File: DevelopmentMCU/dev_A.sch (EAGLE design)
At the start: 9 parts, among them U1 TM4C123_DEVICE

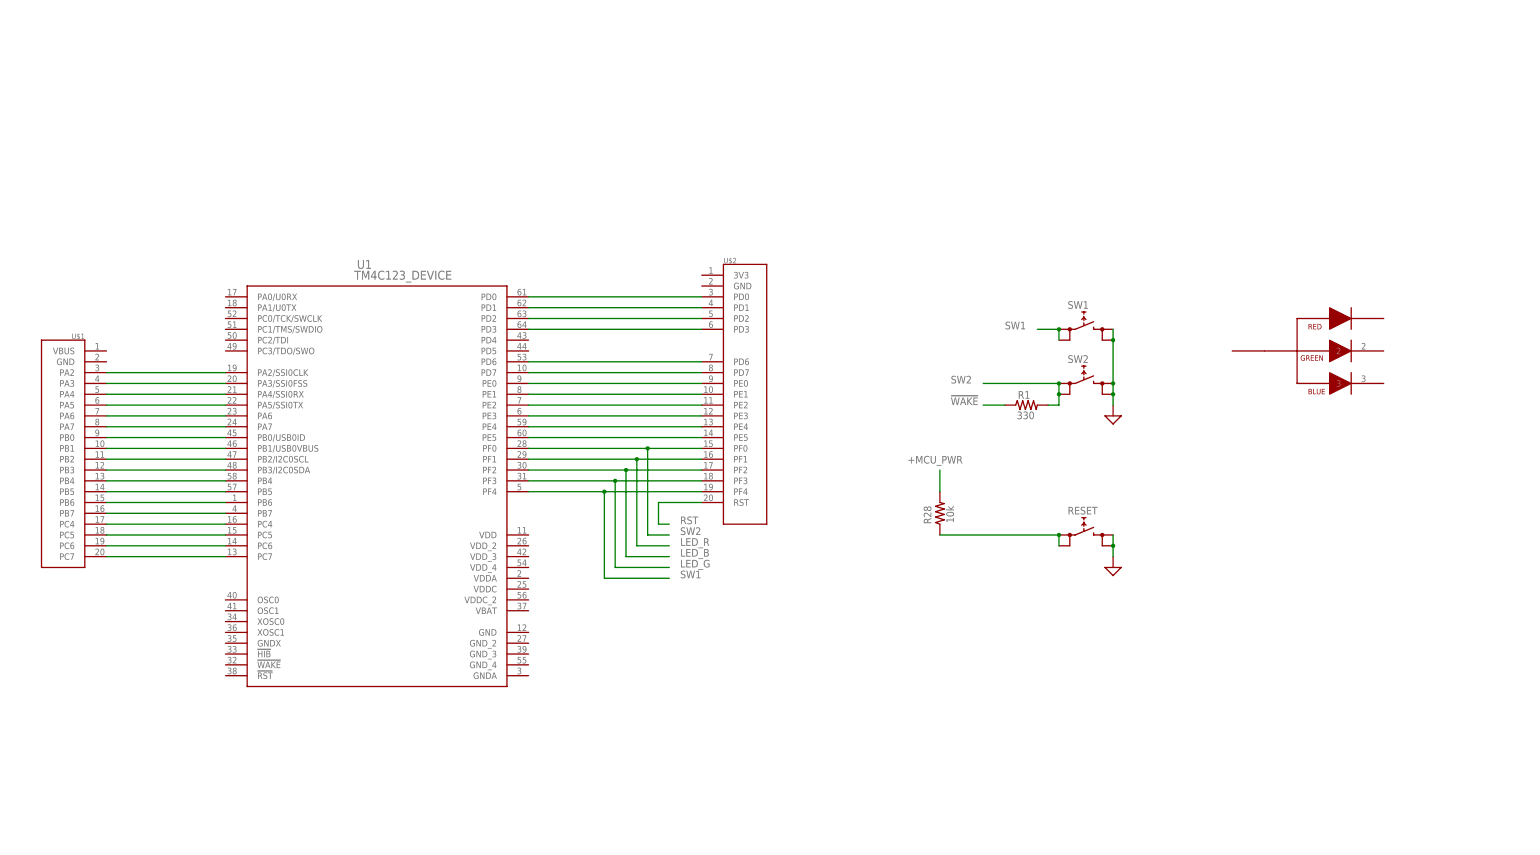
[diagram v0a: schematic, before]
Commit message: Staging
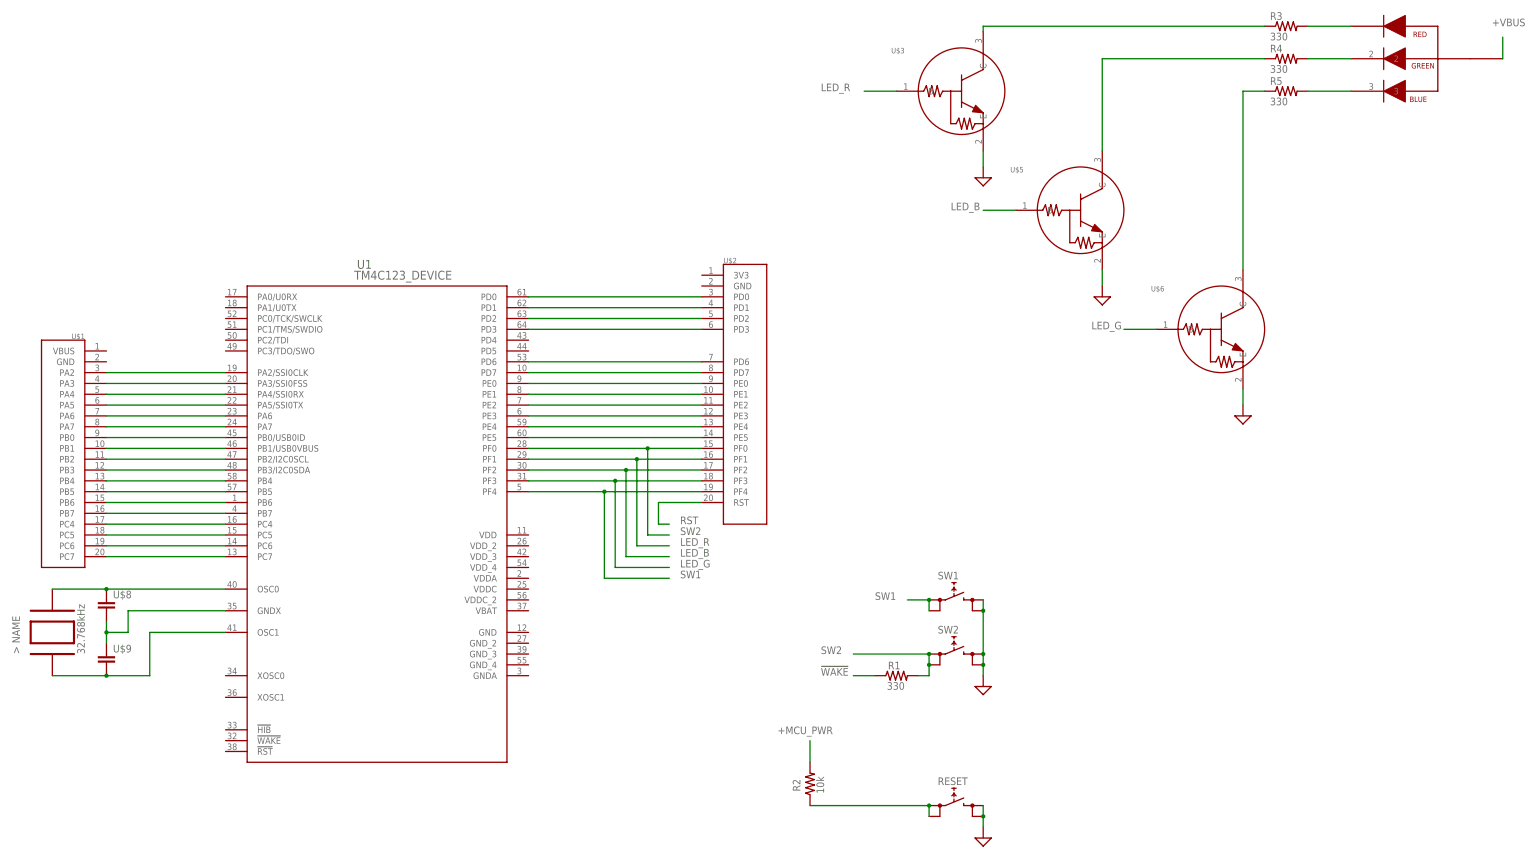
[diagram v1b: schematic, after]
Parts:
- removed R28: 10k, MICROCONTROLLER:RESISTOR
- added R2: 10k, MICROCONTROLLER:RESISTOR
- added R3, R4, R5: 330, MICROCONTROLLER:RESISTOR
- added U$3, U$5, U$6: (no value), MICROCONTROLLER:NPN_BJT
- added U$7: 32kHz, MICROCONTROLLER:32KHZ_OSCILATOR
- added U$8, U$9: (no value), MICROCONTROLLER:CAPACITOR
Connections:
- new net +VBUS: U$4.4
- new net N$32: R3.2, U$4.1
- new net N$33: R4.2, U$4.2
- new net N$34: R5.2, U$4.3
- new net N$35: R5.1, U$6.C
- new net N$36: R4.1, U$5.C
- new net N$37: R3.1, U$3.C
- new net N$38: U$7.2, U$8.1, U1.OSC0
- new net N$39: U$7.1, U$9.2, U1.OSC1
- new net N$40: U$8.2, U$9.1, U1.GNDX
- net +MCU_PWR: now also R2.2; no longer R28.2
- net GND: now also U$3.E, U$5.E, U$6.E
- net LED_B: now also U$5.B
- net LED_G: now also U$6.B
- net LED_R: now also U$3.B
- net N$31: now also R2.1; no longer R28.1
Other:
- moved on the sheet: R1, RESET, SW1, SW2, U1
